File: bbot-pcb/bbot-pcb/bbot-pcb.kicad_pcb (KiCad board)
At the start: 2 copper layers, 63.5 x 52.1 mm, 10 parts, among them U1 HA-552-4P, U3 HA-552-4P

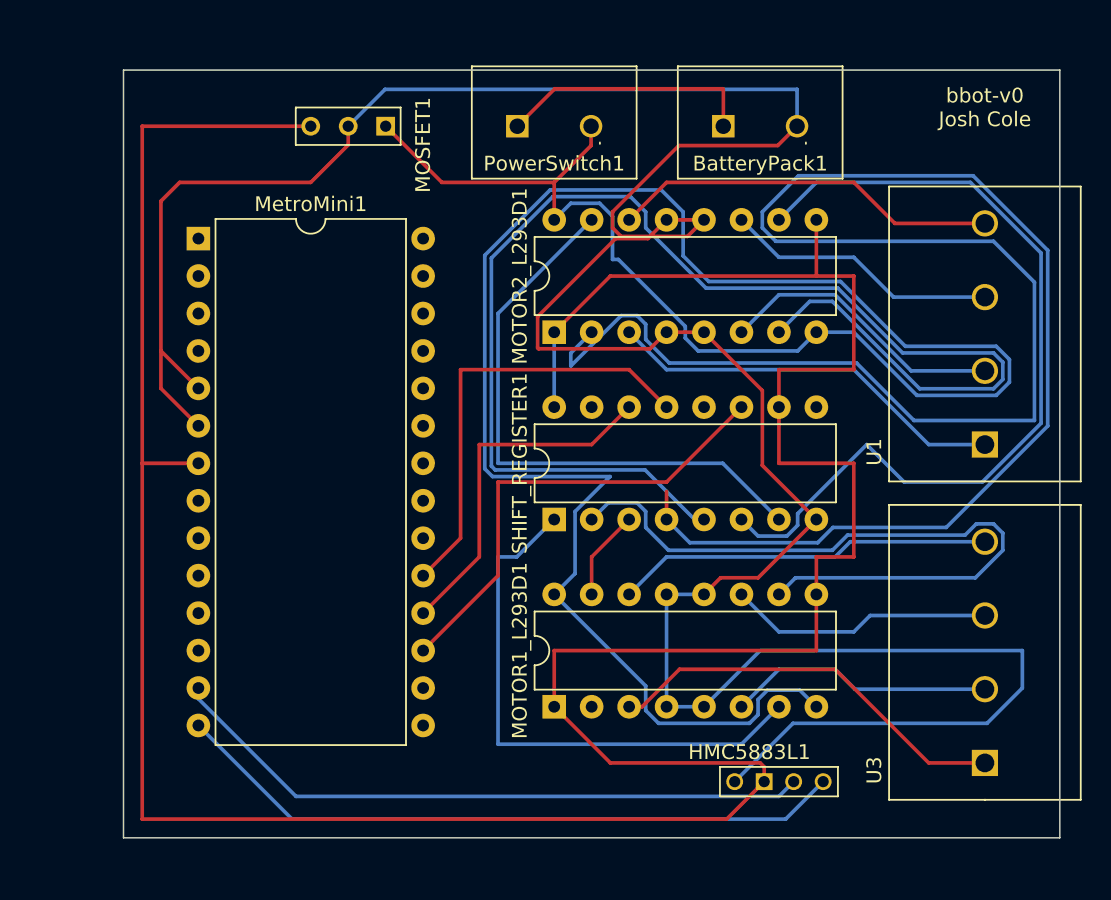
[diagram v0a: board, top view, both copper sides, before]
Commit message: finalize kicad circuit board.
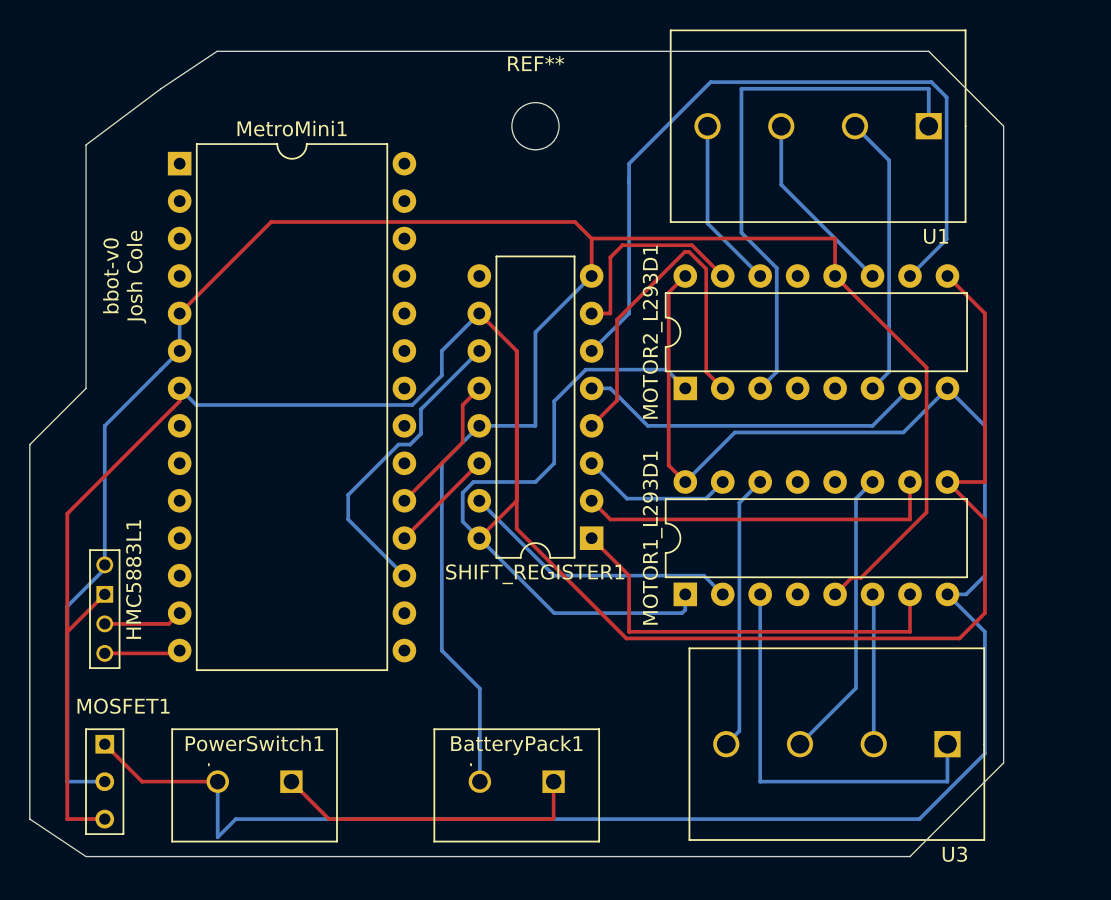
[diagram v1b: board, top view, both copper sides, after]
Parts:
- added REF**: MountingHole_3.2mm_M3, MountingHole:MountingHole_3.2mm_M3, F.Cu at (146.1, 62.2)
- moved PowerSwitch1 48.9 mm to (127.0, 106.7), turned to 180 degrees
- moved BatteryPack1 47.4 mm to (144.8, 106.7), turned to 180 degrees
- moved MOSFET1 47.4 mm to (116.8, 106.7), turned to 270 degrees
- moved HMC5883L1 47.2 mm to (116.8, 95.0), turned to 270 degrees
- moved U1 21.9 mm to (172.7, 62.2), turned to 180 degrees
- moved MOTOR1_L293D1 11.7 mm to (156.2, 94.0)
- moved MOTOR2_L293D1 9.67 mm to (156.2, 80.0)
- moved MetroMini1 5.24 mm to (121.9, 64.8)
- moved SHIFT_REGISTER1 2.84 mm to (149.9, 90.2), turned to 180 degrees
- moved U3 2.84 mm to (174.0, 104.1), turned to 180 degrees
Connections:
- MOTOR1_L293D1 pad 12: GND -> Net-(MOTOR1_L293D1-Pad12)
- MOTOR1_L293D1 pad 13: GND -> Net-(MOTOR1_L293D1-Pad13)
- MOTOR1_L293D1 pad 4: GND -> Net-(MOTOR1_L293D1-Pad4)
- MOTOR2_L293D1 pad 13: GND -> Net-(MOTOR2_L293D1-Pad13)
- MOTOR2_L293D1 pad 4: GND -> Net-(MOTOR2_L293D1-Pad4)
- MOTOR2_L293D1 pad 5: GND -> Net-(MOTOR2_L293D1-Pad5)
- SHIFT_REGISTER1 pad 12: Net-(SHIFT_REGISTER1-Pad12) -> SHIFT_LATCH
- SHIFT_REGISTER1 pad 13: SHIFT_LATCH -> GND
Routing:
- net /MOTOR2_A: track 135.8 -> 24.9 mm
- net /MOTOR2_B: track 91.6 -> 23.7 mm
- net GND: track 206.4 -> 158.9 mm
- net SCL: track 46.1 -> 5.16 mm
- net SDA: track 44.3 -> 5.38 mm
- net /12V: track 163.3 -> 130.8 mm
- net /MOTOR2_D: track 39.8 -> 13.9 mm
- net /MOTOR1_C: track 48.9 -> 24.7 mm
- net SHIFT_LATCH: track 30.0 -> 9.72 mm
- net /MOTOR1_A: track 0.00 -> 19.1 mm
- net SHIFT_DATA: track 24.2 -> 7.18 mm
- net 5V: track 212.9 -> 197.6 mm
- net /MOTOR2_PHASE_D: track 26.3 -> 11.6 mm
- net SHIFT_CLCK: track 32.1 -> 21.0 mm
- net /MOTOR2_PHASE_A: track 27.3 -> 37.0 mm
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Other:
- board size 63.5 x 52.1 mm -> 66 x 54.6 mm
- board text added: "Battery Pack"
- board text added: "Power Switch"
- board text added: "a robot"
- board text added: "is this enough?"
- board text added: "lol"
